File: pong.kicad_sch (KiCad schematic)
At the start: 8 parts, among them U1 L7805

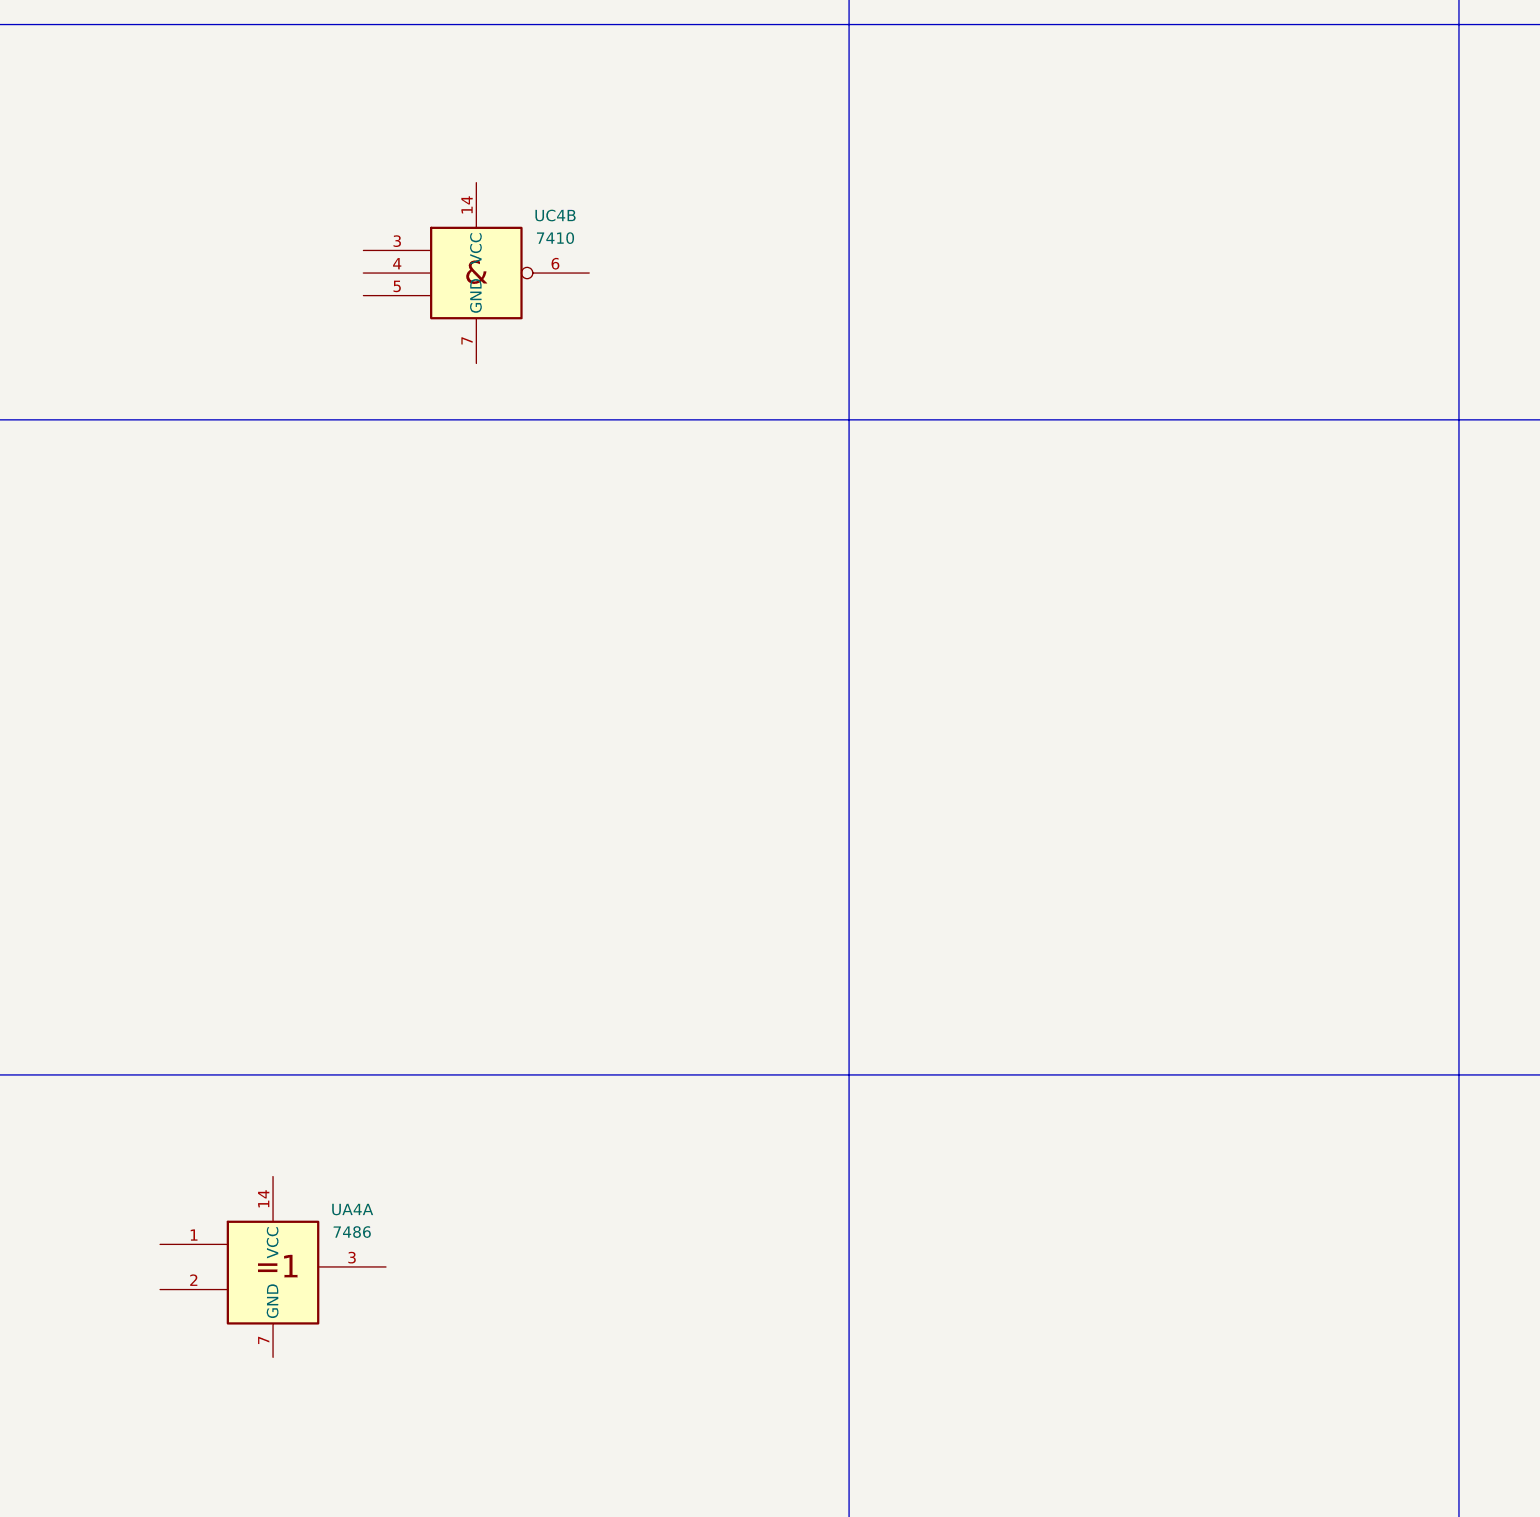
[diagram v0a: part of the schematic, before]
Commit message: R20260922PM
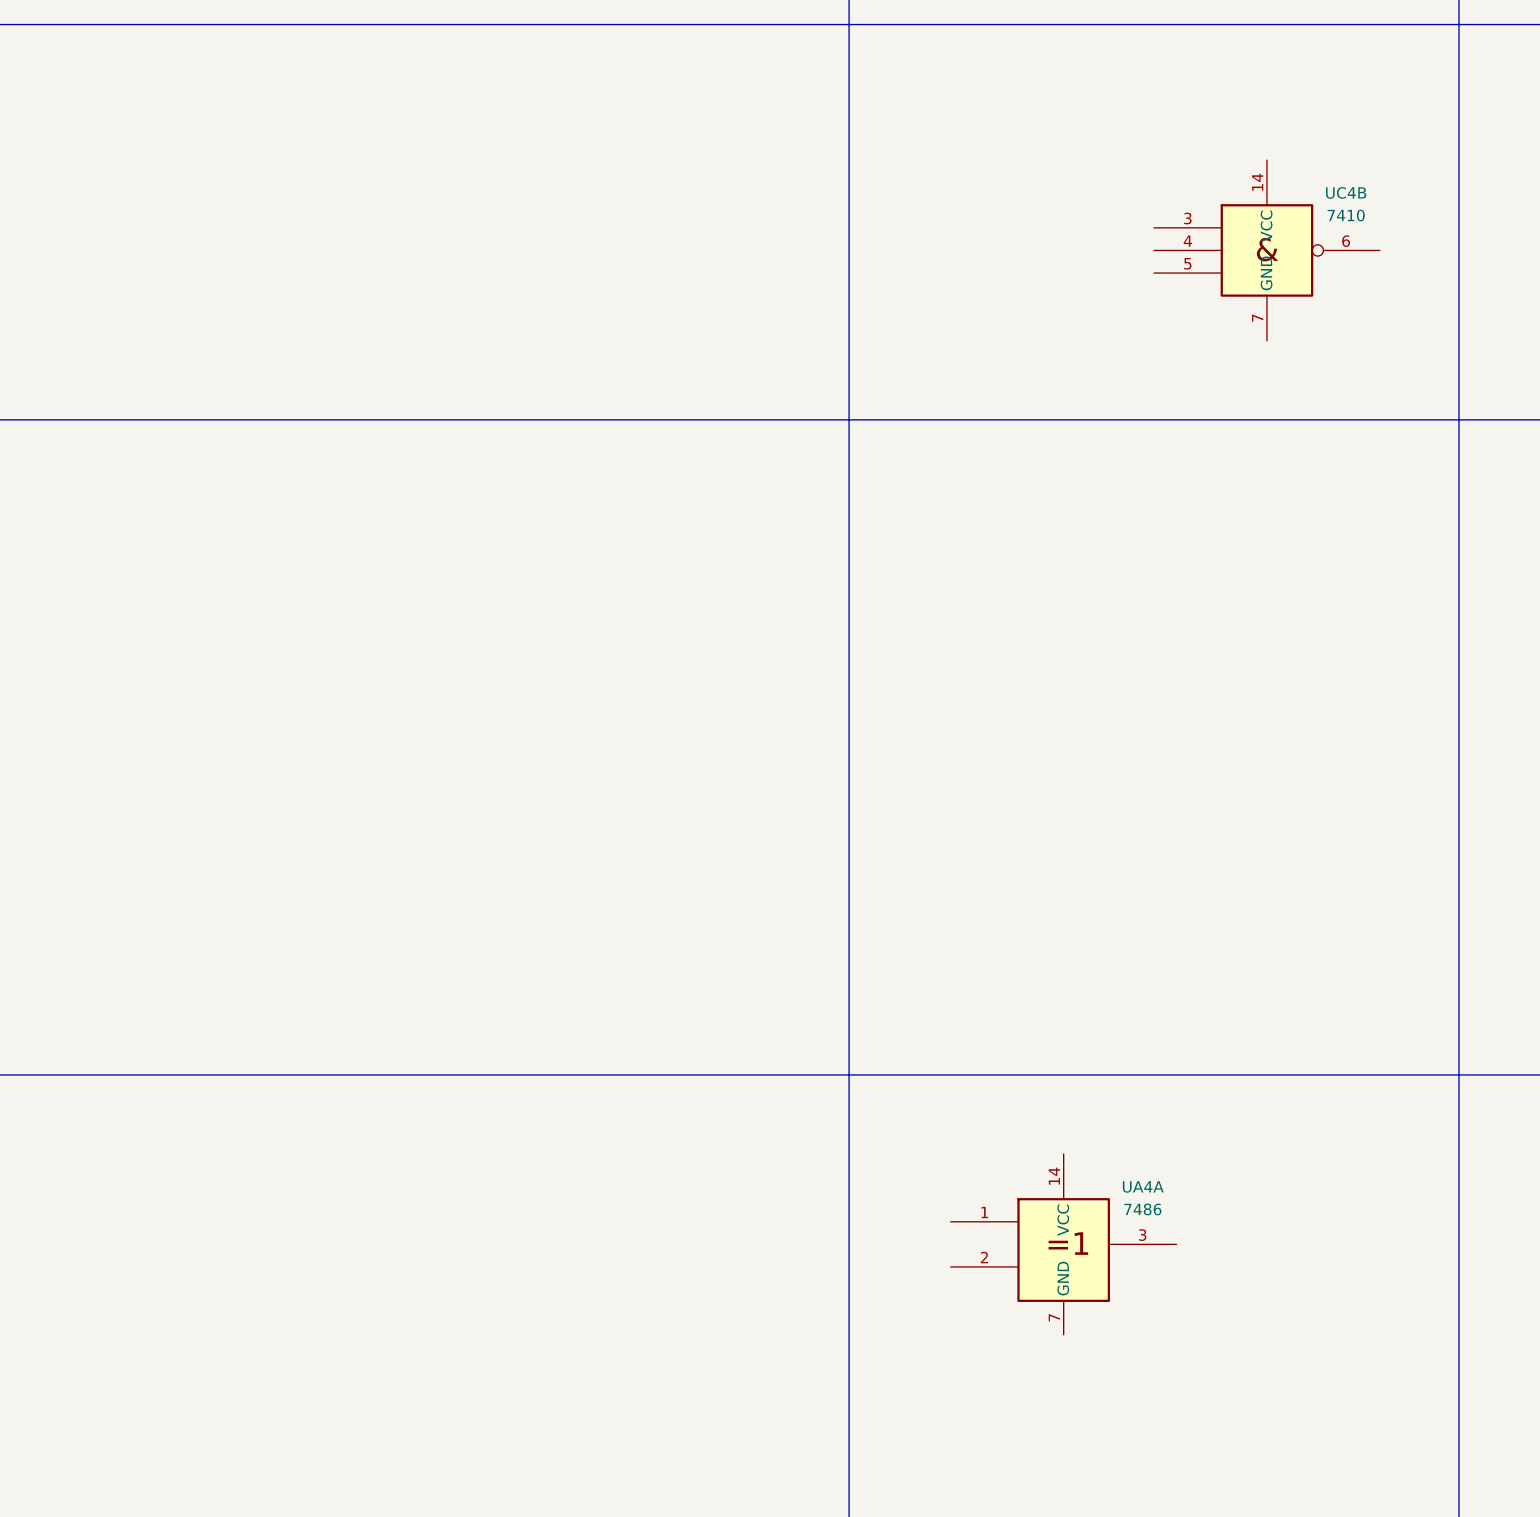
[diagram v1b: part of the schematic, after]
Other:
- moved on the sheet: UA4A, UC4B
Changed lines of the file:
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@@
 	(symbol
 		(lib_id "74xx_IEEE:7410")
-		(at 321.31 -163.83 0)
+		(at 410.21 -166.37 0)
 		(unit 2)
 		(body_style 1)
@@
 		(fields_autoplaced yes)
 		(property "Reference" "UC4"
-			(at 330.2 -170.2502 0)
+			(at 419.1 -172.7902 0)
 			(show_name no)
 			(do_not_autoplace no)
@@
 		)
 		(property "Value" "7410"
-			(at 330.2 -167.7102 0)
+			(at 419.1 -170.2502 0)
 			(show_name no)
 			(do_not_autoplace no)
@@
 		)
 		(property "Footprint" "pong:pong_DIP-14_W7.62mm_Socket_LongPads"
-			(at 321.31 -163.83 0)
+			(at 410.21 -166.37 0)
 			(hide yes)
 			(show_name no)
@@
 		)
 		(property "Datasheet" ""
-			(at 321.31 -163.83 0)
+			(at 410.21 -166.37 0)
 			(hide yes)
 			(show_name no)
@@
 		)
 		(property "Description" ""
-			(at 321.31 -163.83 0)
+			(at 410.21 -166.37 0)
 			(hide yes)
 			(show_name no)
@@
 	(symbol
 		(lib_id "74xx_IEEE:7486")
-		(at 298.45 -52.07 0)
+		(at 387.35 -54.61 0)
 		(unit 1)
 		(body_style 1)
@@
 		(fields_autoplaced yes)
 		(property "Reference" "UA4"
-			(at 307.34 -58.4902 0)
+			(at 396.24 -61.0302 0)
 			(show_name no)
 			(do_not_autoplace no)
@@
 		)
 		(property "Value" "7486"
-			(at 307.34 -55.9502 0)
+			(at 396.24 -58.4902 0)
 			(show_name no)
 			(do_not_autoplace no)
@@
 		)
 		(property "Footprint" "pong:pong_DIP-14_W7.62mm_Socket_LongPads"
-			(at 298.45 -52.07 0)
+			(at 387.35 -54.61 0)
 			(hide yes)
 			(show_name no)
@@
 		)
 		(property "Datasheet" ""
-			(at 298.45 -52.07 0)
+			(at 387.35 -54.61 0)
 			(hide yes)
 			(show_name no)
@@
 		)
 		(property "Description" ""
-			(at 298.45 -52.07 0)
-			(hide yes)
-			(show_name no)
+			(at 387.35 -54.61 0)
+			(hide yes)
+			(show_name no)
